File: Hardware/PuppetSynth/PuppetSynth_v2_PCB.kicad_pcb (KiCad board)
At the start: 2 copper layers, 445.2 x 254.9 mm, 57 parts, among them J1 ADS1115, J11 JST_03, J12 JST_03, J13 JST_05, J14 JST_05, J15 JST_05, J16 JST_03, J17 JST_03, J18 JST_03, J2 ADS1115, J20 JST_03, J21 JST_03, J22 JST_03, J24 JST_03, J25 JST_03, J26 JST_03, J3 JST_03, J4 JST_03, J5 JST_05, J6 JST_05, J7 JST_05

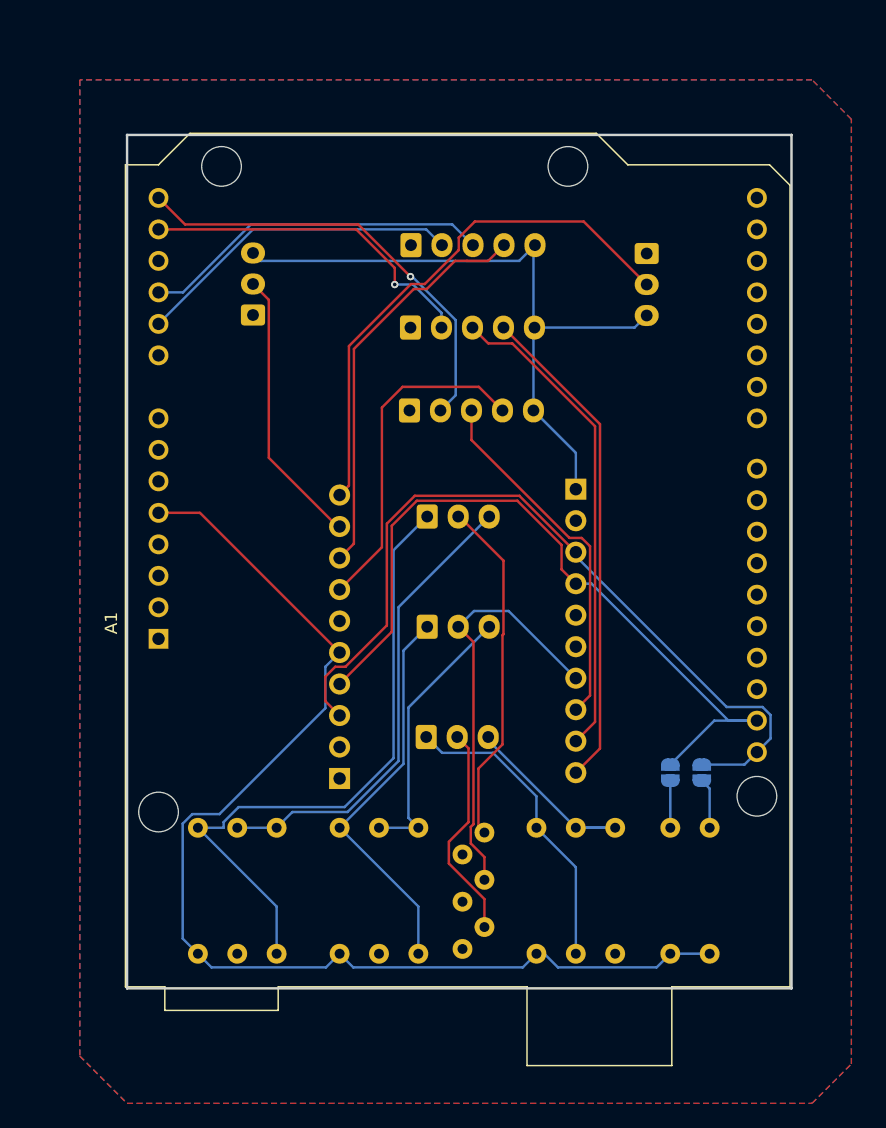
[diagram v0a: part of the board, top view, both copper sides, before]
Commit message: updated pcb
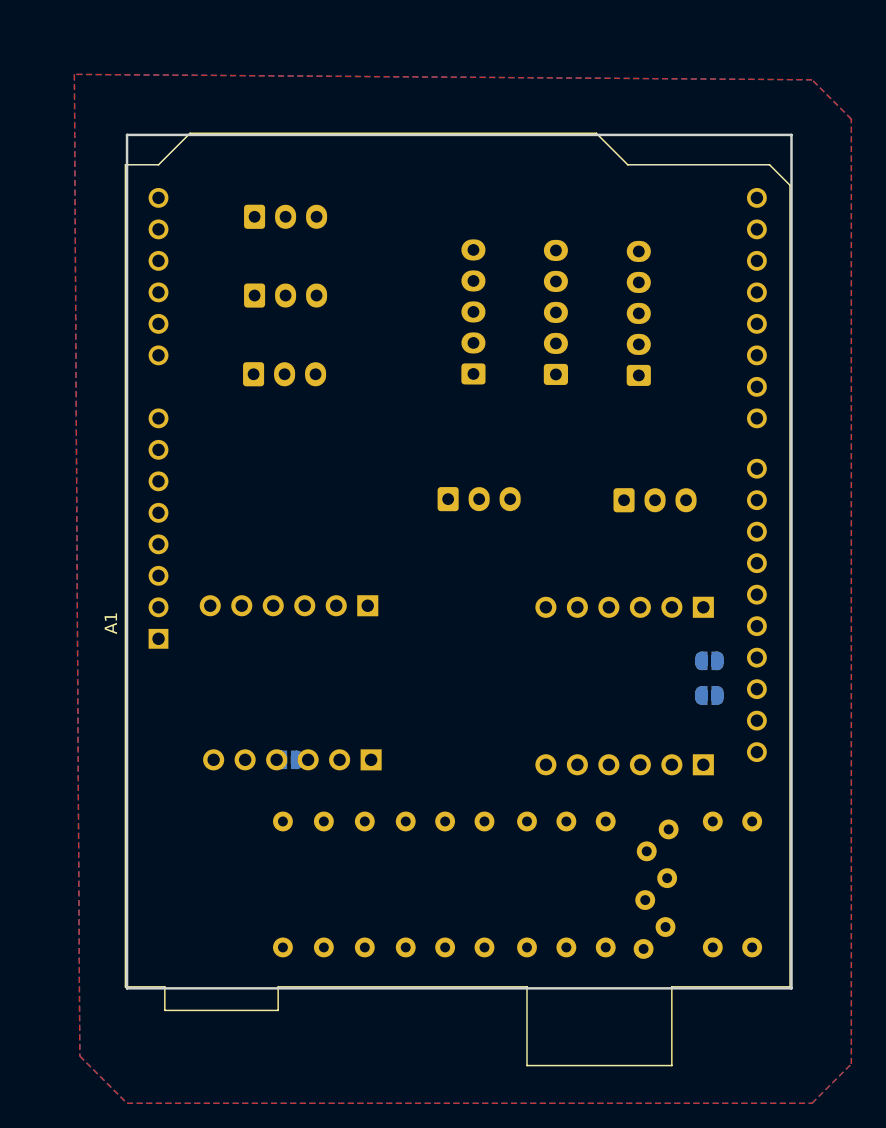
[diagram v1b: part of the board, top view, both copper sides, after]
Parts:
- removed J1, J2: ADS1115, Connector_PinSocket_2.54mm:PinSocket_1x10_P2.54mm_Vertical
- removed the JP2 at (364.5, 337.2)
- added G***: LOGO, LOGO, F.Cu at (347.9, 329.6)
- added G***: LOGO, LOGO, F.Cu at (347.7, 319.7)
- added G***: LOGO, LOGO, B.Cu at (326.1, 346.5)
- added J10: PINHD_1x6_Female, Connector_PinSocket_2.54mm:PinSocket_1x06_P2.54mm_Vertical, B.Cu at (367.2, 336.6)
- added J19: PINHD_1x6_Female, Connector_PinSocket_2.54mm:PinSocket_1x06_P2.54mm_Vertical, B.Cu at (367.2, 323.9)
- added J8: PINHD_1x6_Female, Connector_PinSocket_2.54mm:PinSocket_1x06_P2.54mm_Vertical, B.Cu at (340.4, 336.2)
- added J9: PINHD_1x6_Female, Connector_PinSocket_2.54mm:PinSocket_1x06_P2.54mm_Vertical, B.Cu at (340.1, 323.7)
- added JP2: Jumper_2_Bridged, Jumper:SolderJumper-2_P1.3mm_Open_RoundedPad1.0x1.5mm, B.Cu at (367.6, 328.2)
- added JP2: Jumper_2_Bridged, Jumper:SolderJumper-2_P1.3mm_Open_RoundedPad1.0x1.5mm, B.Cu at (333.7, 336.2)
- A1: footprint Module:Arduino_UNO_R3_WithMountingHoles -> Module:Arduino_UNO_R3
- moved J26 32.4 mm to (330.9, 305.1)
- moved J25 30.1 mm to (331.0, 298.7)
- moved J24 27.9 mm to (331.0, 292.4)
- moved J12 21.6 mm to (346.6, 315.1), turned to 0 degrees
- moved J11 20.0 mm to (360.8, 315.2), turned to 0 degrees
- moved J13 18.7 mm to (361.9, 305.1), turned to 90 degrees
- moved C3 14.9 mm to (364.4, 341.8)
- moved C4 14.7 mm to (364.2, 345.7)
- moved C5 14.6 mm to (364.1, 349.6)
- moved J14 12.3 mm to (355.3, 305.1), turned to 90 degrees
- moved J15 11.5 mm to (348.6, 305.0), turned to 90 degrees
- moved R4 7.13 mm to (339.9, 341.1)
- moved R5 7.00 mm to (336.6, 351.3)
- moved R9 6.88 mm to (333.2, 341.1)
- moved JP1 6.25 mm to (367.6, 331.0), turned to 180 degrees
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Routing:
- net +5V: track 148.7 -> 0.00 mm
- net SCL: track 66.2 -> 0.00 mm
- net SDA: track 61.7 -> 0.00 mm
- net Net-(J24-Pad1): track 51.8 -> 0.00 mm
- net Main_1: track 43.2 -> 0.00 mm
- net Switch_2: track 39.9 -> 0.00 mm
- net Knob_2: track 39.2 -> 0.00 mm
- net Net-(J24-Pad3): track 38.0 -> 0.00 mm
- net Small_Fader_1: track 35.8 -> 0.00 mm, vias 1 -> 0
- net Toggle_2: track 33.7 -> 0.00 mm
- net Switch_3: track 32.9 -> 0.00 mm
- net Net-(J25-Pad1): track 31.9 -> 0.00 mm
- net Knob_1: track 29.1 -> 0.00 mm
- net Knob_3: track 28.3 -> 0.00 mm
- net Net-(C3-Pad1): track 28.1 -> 0.00 mm
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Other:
- board text added: "16-bit ADC"
- board text added: "A+"
- board text added: "A-"
- board text added: "A0"
- board text added: "A1"
- board text added: "A2"
- board text added: "A3"
- board text added: "ADDR"
- board text added: "ALRT"
- board text added: "FX3 FX2 FX1"
- board text added: "GND"
- board text added: "Main 1"
- board text added: "Main 2"
- board text added: "PUPPET SYNTHESIZER PCB by Silvan Roth ZHdK 2025"
- board text added: "Repo"
- board text added: "SCL"
- board text added: "SDA"
- board text added: "VIN"
- board text added: "Wave 1 Wave 2 Wave 3"
- board text removed: "1"
- board text removed: "2"
- board text removed: "3"
- board text removed: "4"
- board text removed: "5"
- board text removed: "Effect 1"
- board text removed: "Effect 2"
- board text removed: "Effect 3"
- board text removed: "SDA SCL"
